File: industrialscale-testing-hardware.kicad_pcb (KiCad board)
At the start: 2 copper layers, 68 x 39.5 mm, 19 parts, among them J1 Conn_01x01, J2 Conn_01x01, J3 Conn_01x01, J4 Conn_01x01, J5 Conn_01x01, J6 Conn_01x01, J7 Conn_02x08_Odd_Even, J8 Conn_01x01, J9 Conn_01x01, Q1 AO3400A, Q2 AO3400A

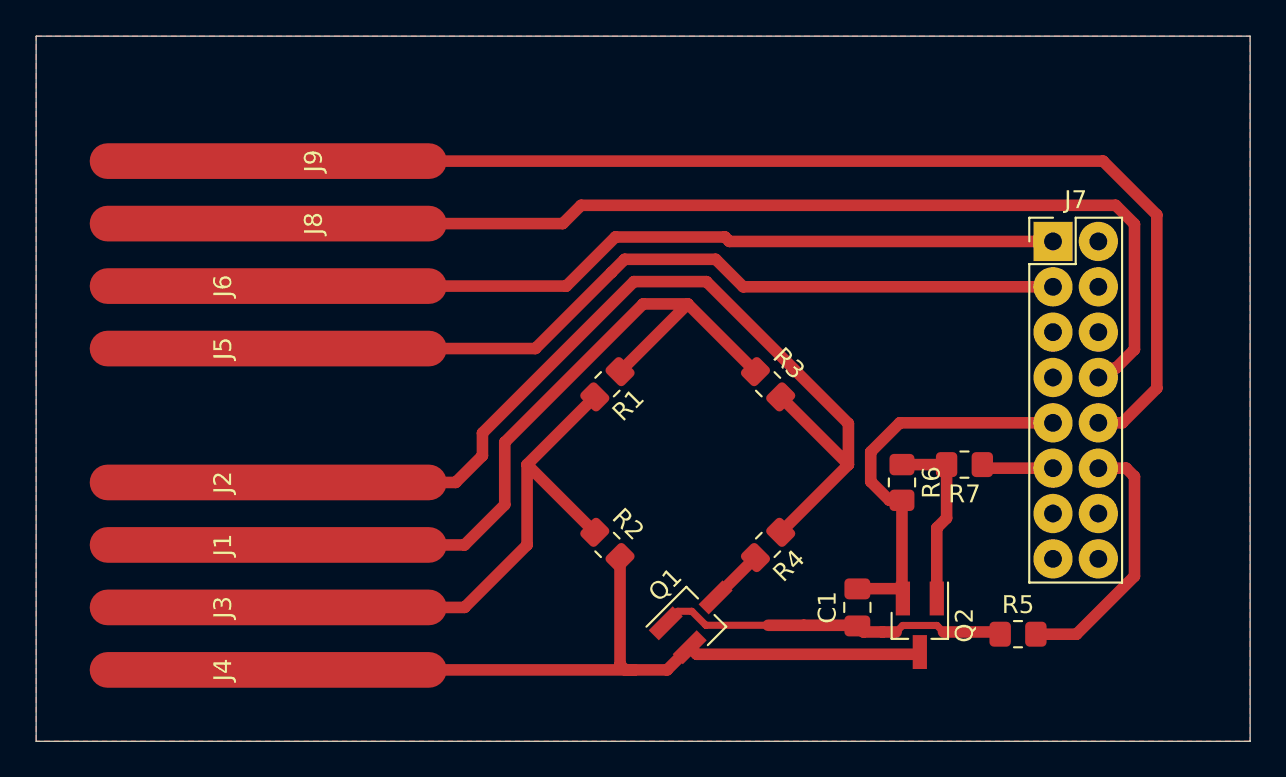
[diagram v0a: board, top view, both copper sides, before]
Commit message: oshpark version
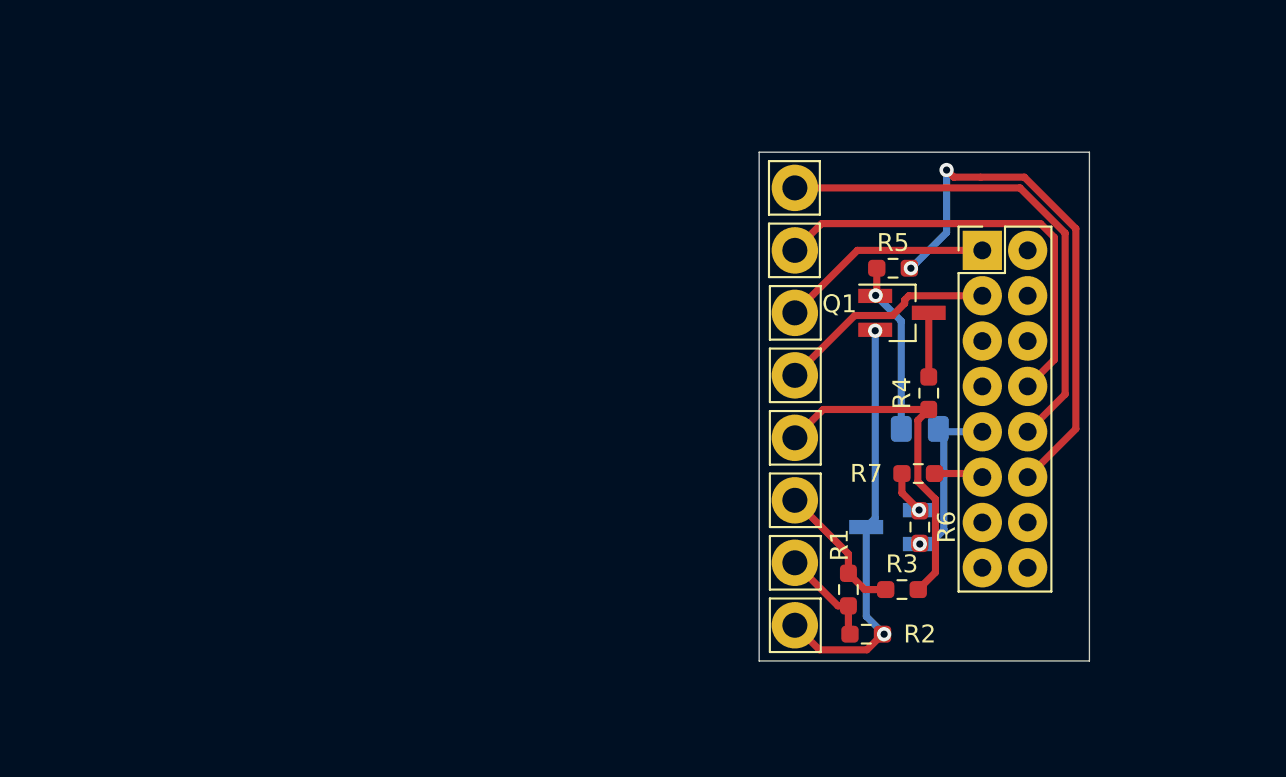
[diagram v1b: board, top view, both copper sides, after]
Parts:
- C1, Q2: moved to B.Cu
- J1, J2, J3, J4, J5, J6, J8, J9: footprint industrialscale-testing-hardware:SolderWirePad_1x01_SMD_2x20mm -> Connector_Pin:Pin_D1.4mm_L8.5mm_W2.8mm_FlatFork
- R1, R2, R3, R4, R5, R6, R7: footprint Resistor_SMD:R_0805_2012Metric_Pad1.20x1.40mm_HandSolder -> Resistor_SMD:R_0603_1608Metric_Pad0.98x0.95mm_HandSolder
- moved J1 29.6 mm to (140.0, 72.5)
- moved J2 29.6 mm to (140.0, 69.0)
- moved J3 29.6 mm to (140.0, 76.0)
- moved J4 29.6 mm to (140.0, 79.5)
- moved J5 29.5 mm to (140.0, 65.5)
- moved J6 29.5 mm to (140.0, 62.0)
- moved J8 29.5 mm to (140.0, 58.5)
- moved J9 29.5 mm to (140.0, 55.0)
- moved R5 21.7 mm to (145.5, 59.5)
- moved Q1 20.5 mm to (146.0, 62.0), turned to 0 degrees
- moved R1 17.7 mm to (143.0, 77.5), turned to 270 degrees
- moved R2 15.3 mm to (144.0, 80.0), turned to 0 degrees
- moved R3 13.7 mm to (146.0, 77.5), turned to 0 degrees
- moved R4 12.4 mm to (147.5, 66.5), turned to 90 degrees
- moved C1 10.6 mm to (147.0, 68.5), turned to 0 degrees
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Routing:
- net APOS: track 61.7 -> 19.3 mm
- net /RXD: track 64.4 -> 28.2 mm
- net /TXD: track 58.7 -> 24.4 mm
- net /BOOTMODE: track 46.2 -> 12.5 mm
- net +3V3: track 41.4 -> 7.80 mm
- net Net-(J6-Pad1): track 44.8 -> 11.9 mm
- net ANEG: track 30.7 -> 5.62 mm
- net SWGND: track 43.7 -> 23.5 mm, vias 0 -> 2
- net RPI_PWM: track 14.7 -> 30.0 mm, vias 0 -> 2
- net GND: track 22.2 -> 9.99 mm, vias 0 -> 1
- net Net-(C1-Pad1): track 19.8 -> 9.66 mm, vias 0 -> 1
- net Net-(Q2-Pad1): track 10.2 -> 2.50 mm, vias 0 -> 1
- net Net-(J7-Pad11): track 4.16 -> 2.76 mm
- removed copper zone on F.Cu, net (none)
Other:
- board size 68 x 39.5 mm -> 18.5 x 28.5 mm
- net class Default: clearance 0.6 -> 0.2; trace_width 0.65 -> 0.4
- rule trace_clearance: 0.6 -> 0.2
